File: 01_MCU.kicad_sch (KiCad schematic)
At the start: 59 parts, among them J1 Conn_01x05, J2 Conn_01x03, Q1 PMBT2222A, SW1 SW_SPDT_312, U1 UM803RS, U2 MIMXRT1011DAE5A, Y1 24MHz, Y2 32.768KHz

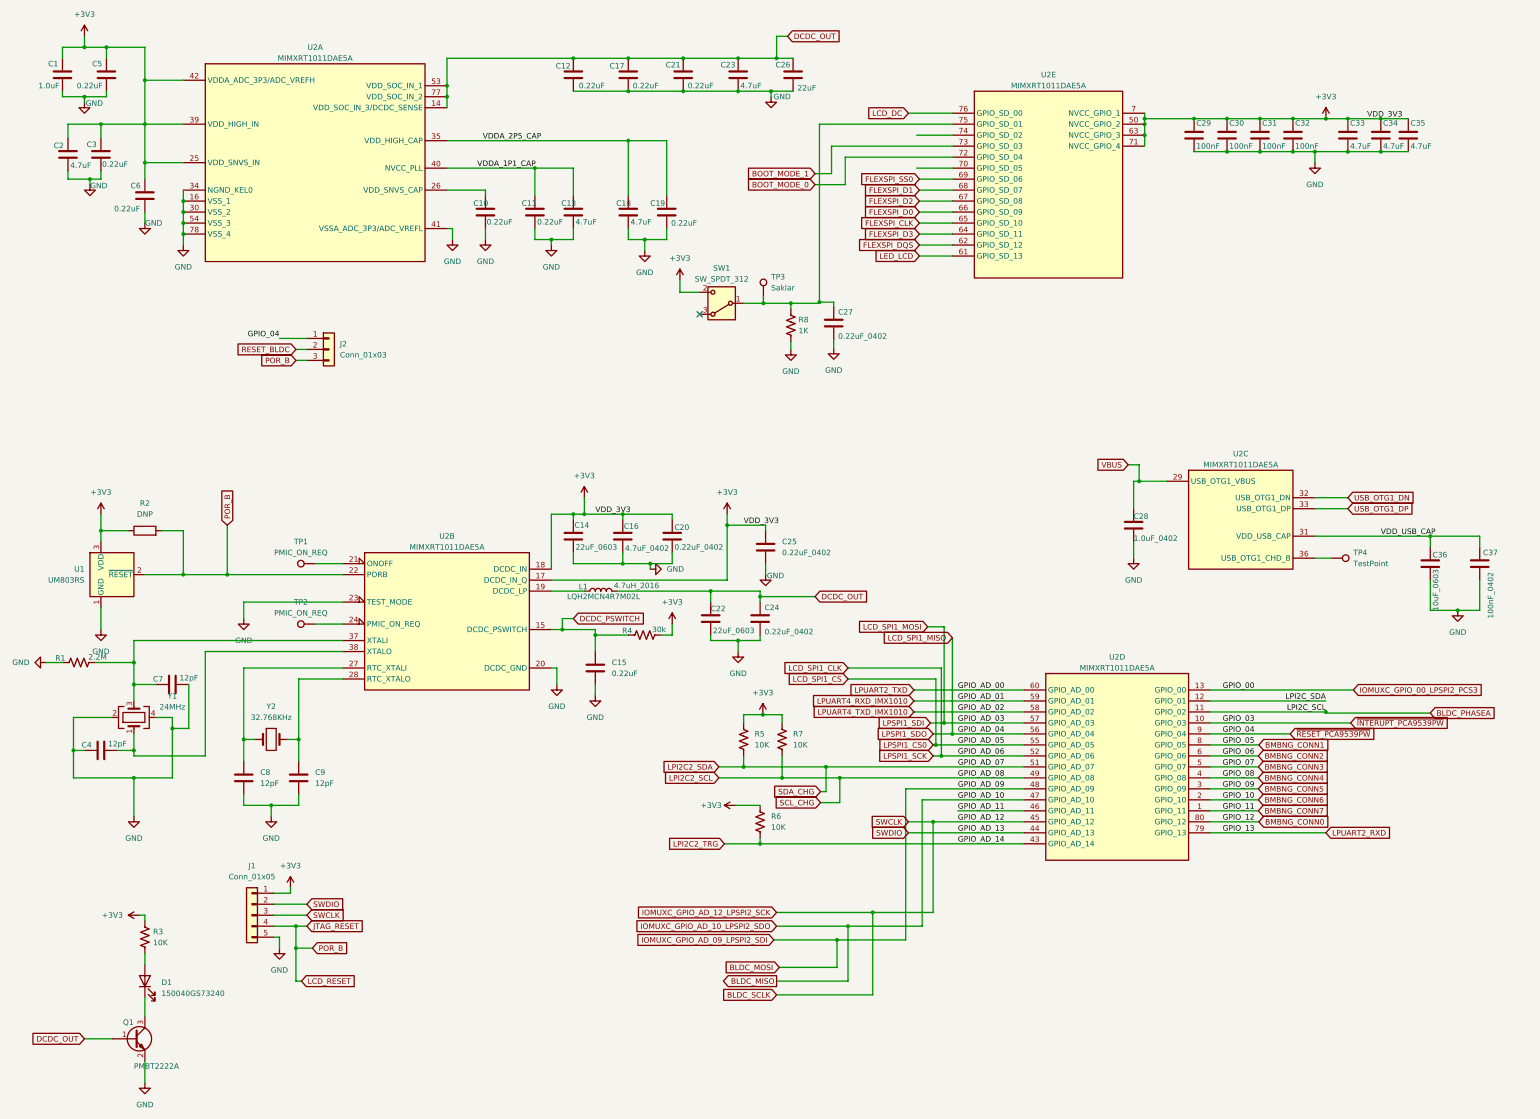
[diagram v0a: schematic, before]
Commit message: dad
da
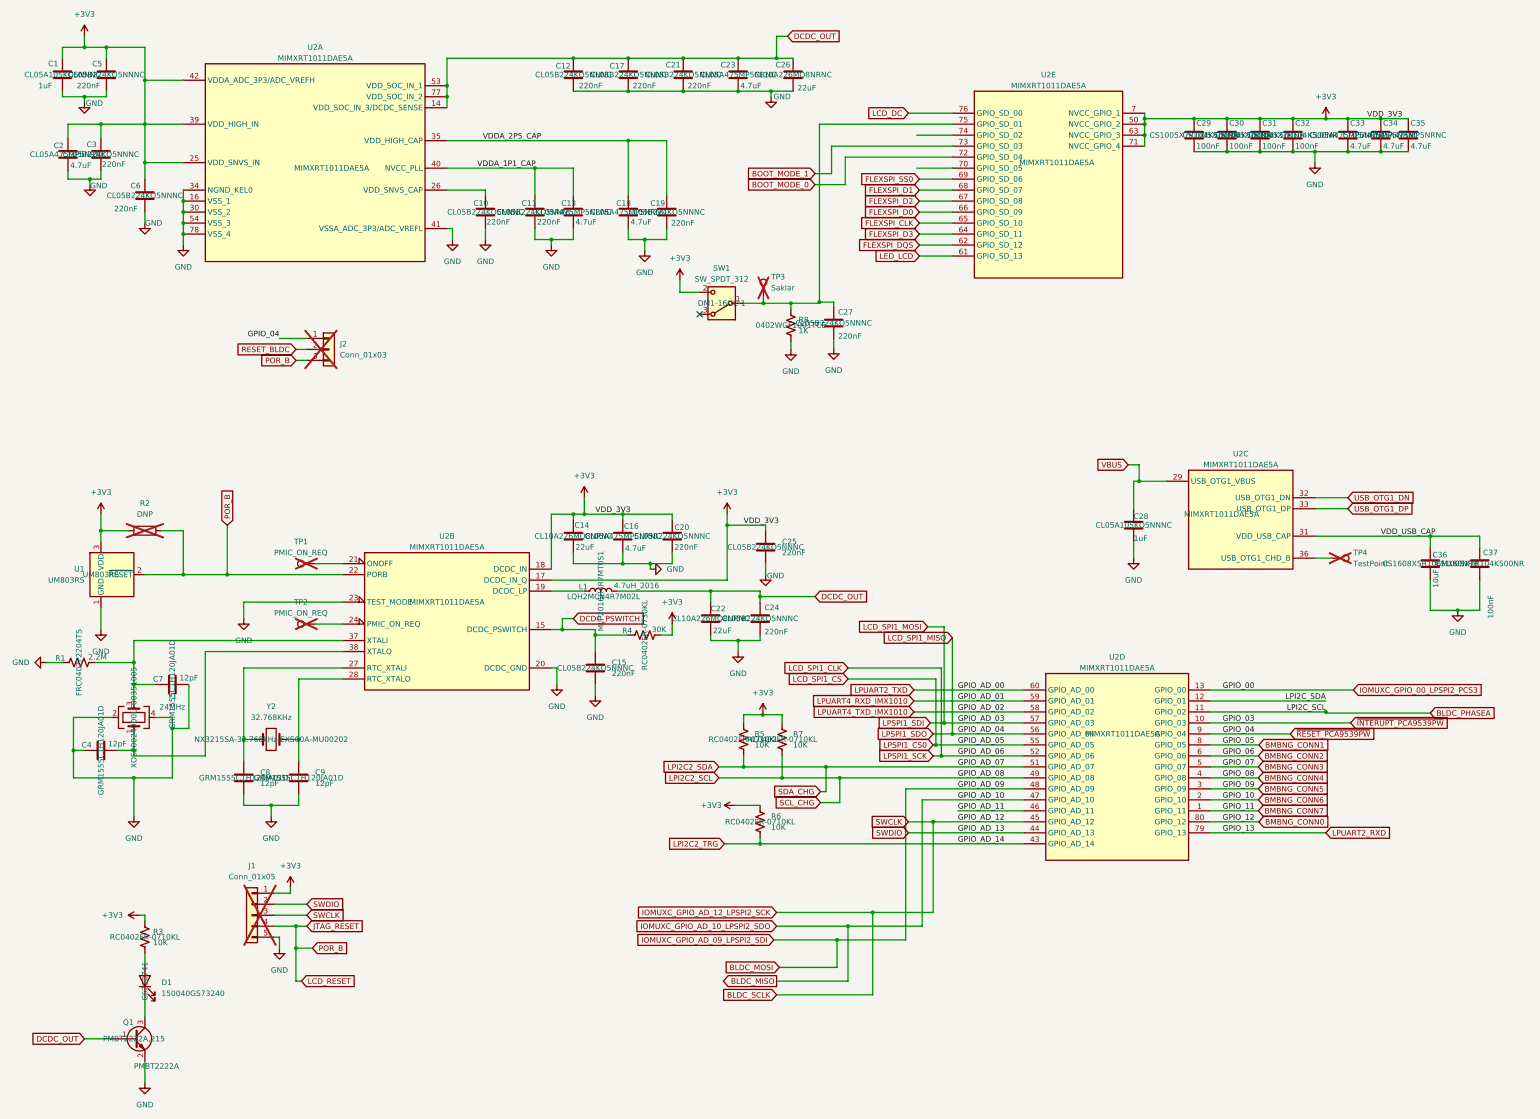
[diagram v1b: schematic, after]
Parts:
- C1: value 1.0uF -> 1uF; Manufacturer_Part_Number (none) -> CL05A105KO5NNNC
- C10, C11, C12, C15, C17, C19, C21, C3, C5, C6: value 0.22uF -> 220nF; Manufacturer_Part_Number (none) -> CL05B224KO5NNNC
- C13, C18, C2, C23, C33, C34, C35: Manufacturer_Part_Number (none) -> CL05A475MP5NRNC
- C14, C22: value 22uF_0603 -> 22uF; Manufacturer_Part_Number (none) -> CL10A226MQ8NRNC
- C16: value 4.7uF_0402 -> 4.7uF; Manufacturer_Part_Number (none) -> CL05A475MP5NRNC
- C20, C24, C25, C27: value 0.22uF_0402 -> 220nF; Manufacturer_Part_Number (none) -> CL05B224KO5NNNC
- C26: Manufacturer_Part_Number (none) -> CL10A226MQ8NRNC
- C28: value 1.0uF_0402 -> 1uF; Manufacturer_Part_Number (none) -> CL05A105KO5NNNC
- C29, C30, C31, C32: Manufacturer_Part_Number (none) -> CS1005X7R104K500NR
- C36: value 10uF_0603 -> 10uF; Manufacturer_Part_Number (none) -> CS1608X5R106M160NRB
- C37: value 100nF_0402 -> 100nF; Manufacturer_Part_Number (none) -> CS1005X7R104K500NR
- C4, C7, C8, C9: Manufacturer_Part_Number (none) -> GRM1555C1H120JA01D
- D1: Manufacturer_Part_Number (none) -> C6210741
- J1, J2, R2, TP1, TP2, TP3, TP4: now not fitted
- L1: Manufacturer_Part_Number (none) -> MLP2016H4R7MT0S1
- Q1: Manufacturer_Part_Number (none) -> PMBT2222A,215
- R1: Manufacturer_Part_Number (none) -> FRC0402F2204TS
- R3, R5, R6, R7: Manufacturer_Part_Number (none) -> RC0402FR-0710KL
- R4: value 30k -> 30K; Manufacturer_Part_Number (none) -> RC0402FR-0730KL
- R8: Manufacturer_Part_Number (none) -> 0402WGF1001TCE
- SW1: Manufacturer_Part_Number (none) -> DM1-16UC-1
- U1: Manufacturer_Part_Number (none) -> UM803RS
- U2: Manufacturer_Part_Number (none) -> MIMXRT1011DAE5A
- Y1: Manufacturer_Part_Number (none) -> XOS20024000LT00351005
- Y2: Manufacturer_Part_Number (none) -> NX3215SA-32.768kHz-EXS00A-MU00202
